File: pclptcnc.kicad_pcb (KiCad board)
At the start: 2 copper layers, 174.8 x 59.1 mm, 250 parts, among them P1 ARK825A-3, P3 ARK825A-4, P4 ARK825A-3, P5 ARK825A-3, P6 ARK825A-3, P7 ARK825A-3, P8 ARK825A-3, Q1 BC807-40, Q10 BC807-40, Q11 BC807-40, Q12 BC807-40, Q13 BC807-40, Q14 BC807-40, Q15 BC807-40, Q16 BC807-40, Q17 BC807-40, Q18 BC807-40, Q2 BC807-40, Q3 BC807-40, Q4 BC807-40, Q5 BC807-40, Q6 BC807-40, Q7 BC807-40, Q8 BC807-40, Q9 BC807-40, U1 74LVC1G3157GW, U10 SN74LVC2G17, U11 74HCT14, U12 SN74LVC2G17, U13 74HCT14, U2 HCPL2630, U3 HCPL2630, U4 HCPL2630, U5 HCPL2630, U6 HCPL2630, U7 HCPL2630, U8 74HCT14, U9 74HCT14, j1 DB25, j2 DB25

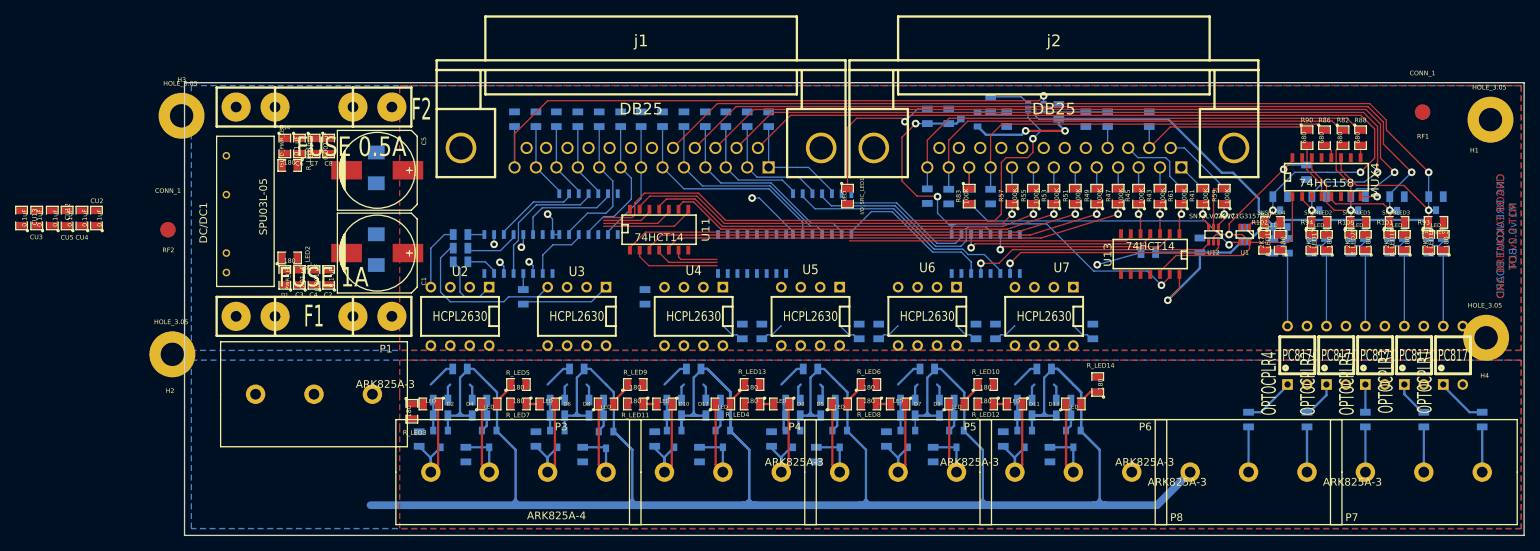
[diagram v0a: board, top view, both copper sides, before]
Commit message: близкая компоновка
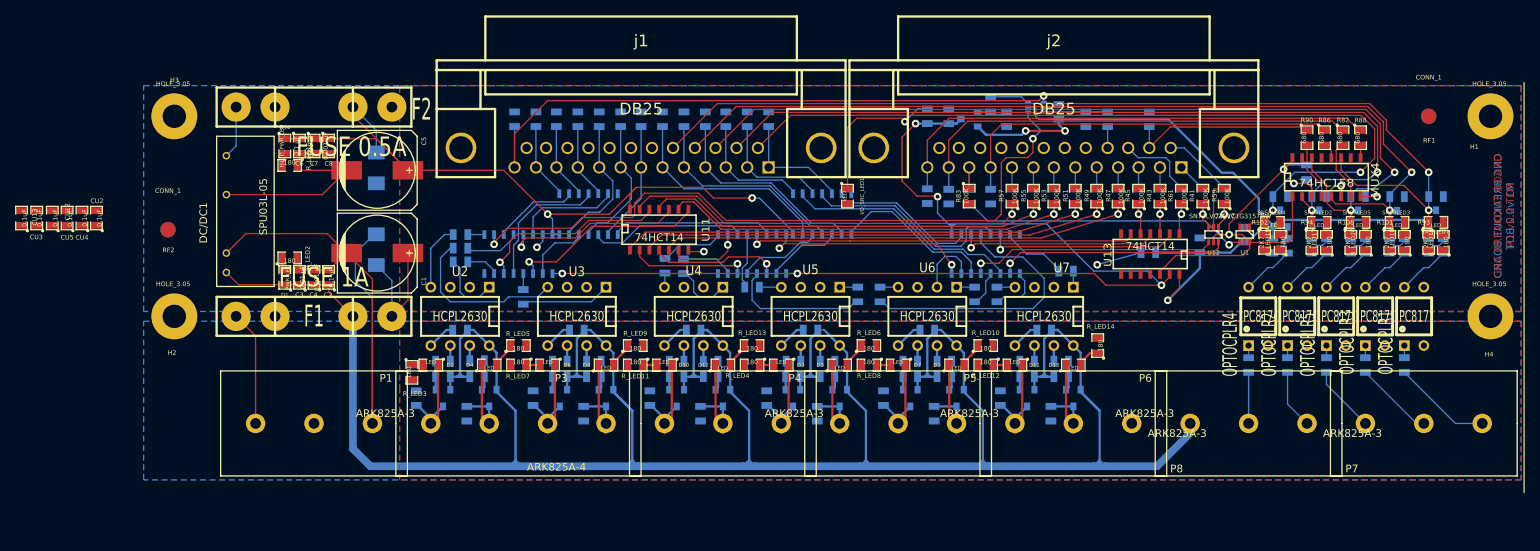
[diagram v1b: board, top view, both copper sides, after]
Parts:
- moved R91 12.4 mm to (194.1, 78.1)
- moved R27 11.5 mm to (100.1, 65.2)
- moved R99 10.4 mm to (189.0, 78.1)
- moved R107 8.74 mm to (184.0, 78.1)
- moved R69 8.61 mm to (150.0, 65.8), turned to 0 degrees
- moved R92 7.55 mm to (178.9, 78.1)
- moved OPTOCPLR1 7.18 mm to (194.1, 75.6)
- moved OPTOCPLR4 7.18 mm to (173.8, 75.6)
- moved OPTOCPLR5 7.18 mm to (184.0, 75.6)
- moved OPTOCPLR2 7.18 mm to (178.9, 75.6)
- moved OPTOCPLR3 7.18 mm to (189.0, 75.6)
- moved R100 7.11 mm to (173.8, 78.1)
- moved P3 6.35 mm to (67.1, 85.7)
- moved P4 6.35 mm to (97.6, 85.7)
- moved P5 6.35 mm to (120.5, 85.7)
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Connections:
- MUX2 pad 11: /RC11 -> /RC7
- MUX2 pad 12: /FLTRD_SGNL6 -> /FLTRD_SGNL7
- MUX2 pad 13: /PC7 -> /PC5
- MUX2 pad 14: /RC7 -> /RC6
- MUX2 pad 2: /RC6 -> /RC11
- MUX2 pad 3: /PC6 -> /PC7
- MUX2 pad 4: /FLTRD_SGNL5 -> /FLTRD_SGNL8
- MUX2 pad 6: /PC5 -> /PC6
- MUX2 pad 7: /FLTRD_SGNL7 -> /FLTRD_SGNL6
- MUX2 pad 9: /FLTRD_SGNL8 -> /FLTRD_SGNL5
- MUX3 pad 7: /FLTRD_SGNL11 -> /FLTRD_SGNL12
- MUX3 pad 9: /FLTRD_SGNL12 -> /FLTRD_SGNL11
- U10 pad 4: /PC12 -> /PC4
- U11 pad 2: /PC4 -> /PC6
- U11 pad 6: /PC6 -> /PC12
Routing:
- net VCC: track 159.4 -> 275.5 mm, vias 7 -> 9
- net /PC/RC_SW: track 60.8 -> 144.8 mm, vias 3 -> 5
- net /PC4: track 12.7 -> 90.8 mm, vias 1 -> 2
- net /ISOLATED_GND: track 22.2 -> 99.3 mm
- net /PC12: track 73.7 -> 10.0 mm
- net /ISOLATED_VCC: track 559.1 -> 620.7 mm
- net GND: track 14.4 -> 65.9 mm, vias 2 -> 6
- net /FLTRD_SGNL9: track 0.00 -> 36.1 mm
- net /RC6: track 0.00 -> 21.1 mm
- net /RC7: track 0.00 -> 20.4 mm
- net /FLTRD_SGNL8: track 0.00 -> 18.4 mm
- net /PC3: track 8.47 -> 25.1 mm
- net /ISOLATED_VCC_NFused: track 0.00 -> 15.0 mm
- net /PC5: track 37.3 -> 50.9 mm, vias 0 -> 1
- net /PC1: track 11.3 -> 23.6 mm
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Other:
- board outline removed

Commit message: version 0.2a completed
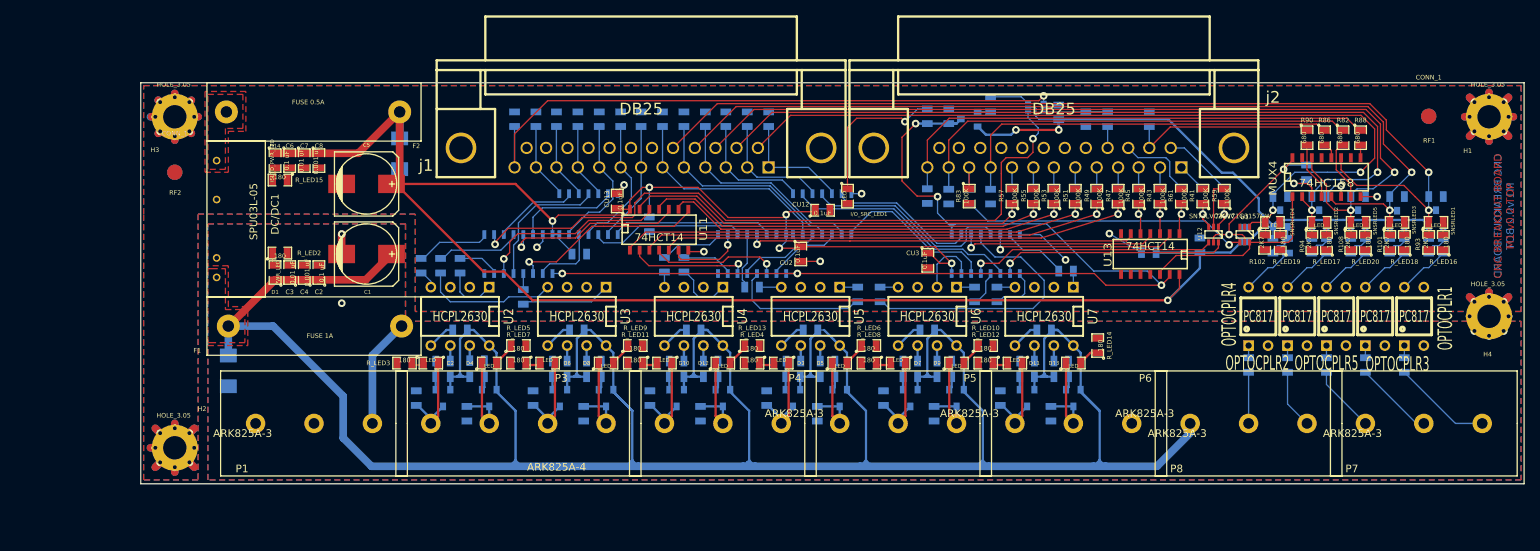
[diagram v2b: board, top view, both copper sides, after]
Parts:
- removed R1: 2K7, SM0805
- C1, C5: footprint c_elec_10x10 -> c_elec_8x10.5
- CU4, CU5: moved to B.Cu
- F1, F2: footprint FUSE5-20_1.4mm -> FUSE_HOLDER
- moved CU4 159.9 mm to (181.4, 53.0), turned to 270 degrees
- moved CU5 153.6 mm to (173.3, 61.1)
- moved CU3 116.4 mm to (132.0, 64.5), turned to 270 degrees
- moved CU12 100.5 mm to (118.2, 57.9), turned to 0 degrees
- moved CU2 92.0 mm to (115.4, 63.6), turned to 270 degrees
- moved CU13 77.7 mm to (91.4, 56.7)
- moved CU15 71.9 mm to (95.6, 59.8), turned to 270 degrees
- moved CU1 65.2 mm to (86.5, 63.6), turned to 0 degrees
- moved TVS1 25.0 mm to (40.7, 78.9), turned to 90 degrees
- moved CU14 21.7 mm to (149.0, 45.1), turned to 90 degrees
- moved H2 17.1 mm to (33.7, 88.9)
- moved CU16 16.9 mm to (167.4, 62.5), turned to 90 degrees
- moved P1 15.2 mm to (59.5, 85.7), turned to 180 degrees
- moved CU17 12.7 mm to (160.8, 63.4), turned to 180 degrees
- moved F1 11.5 mm to (63.3, 73.0), turned to 180 degrees
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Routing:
- net GND: track 65.9 -> 391.3 mm, vias 6 -> 42
- net VCC: track 275.5 -> 395.6 mm, vias 9 -> 10
- net /ISOLATED_GND: track 99.3 -> 24.8 mm, vias 0 -> 1
- net /FLTRD_SGNL1: track 2.16 -> 9.87 mm
- net /VCC_NFused: track 6.88 -> 0.00 mm
- net N-00000138: track 8.74 -> 2.48 mm
- net /ISOLATED_VCC: track 620.7 -> 626.3 mm
- net N-00000174: track 21.9 -> 17.5 mm
- net /FLTRD_SGNL3: track 7.19 -> 11.1 mm
- net /IOSRCTR_BASE: track 4.56 -> 1.69 mm
- net N-00000137: track 8.90 -> 6.82 mm
- net /FLTRD_SGNL2: track 4.28 -> 5.48 mm
- net /OUTPUT_SIGNAL9: track 14.8 -> 13.8 mm
- net /OUTPUT_SIGNAL8: track 14.6 -> 13.6 mm
- net /OUTPUT_SIGNAL7: track 15.4 -> 14.4 mm
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- added copper zone on F.Cu, net /ISOLATED_VCC
- added copper zone on F.Cu, net /VCC_NFused
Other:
- board outline added: 180.5 x 52.3 mm
